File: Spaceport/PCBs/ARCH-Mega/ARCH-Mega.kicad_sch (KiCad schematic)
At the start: 83 parts, among them J10 USB_C_Receptacle_USB2.0_16P, J12 Charge, U4 FT234XD, U5 USBLC6-2P6, U8 BQ25606RGER

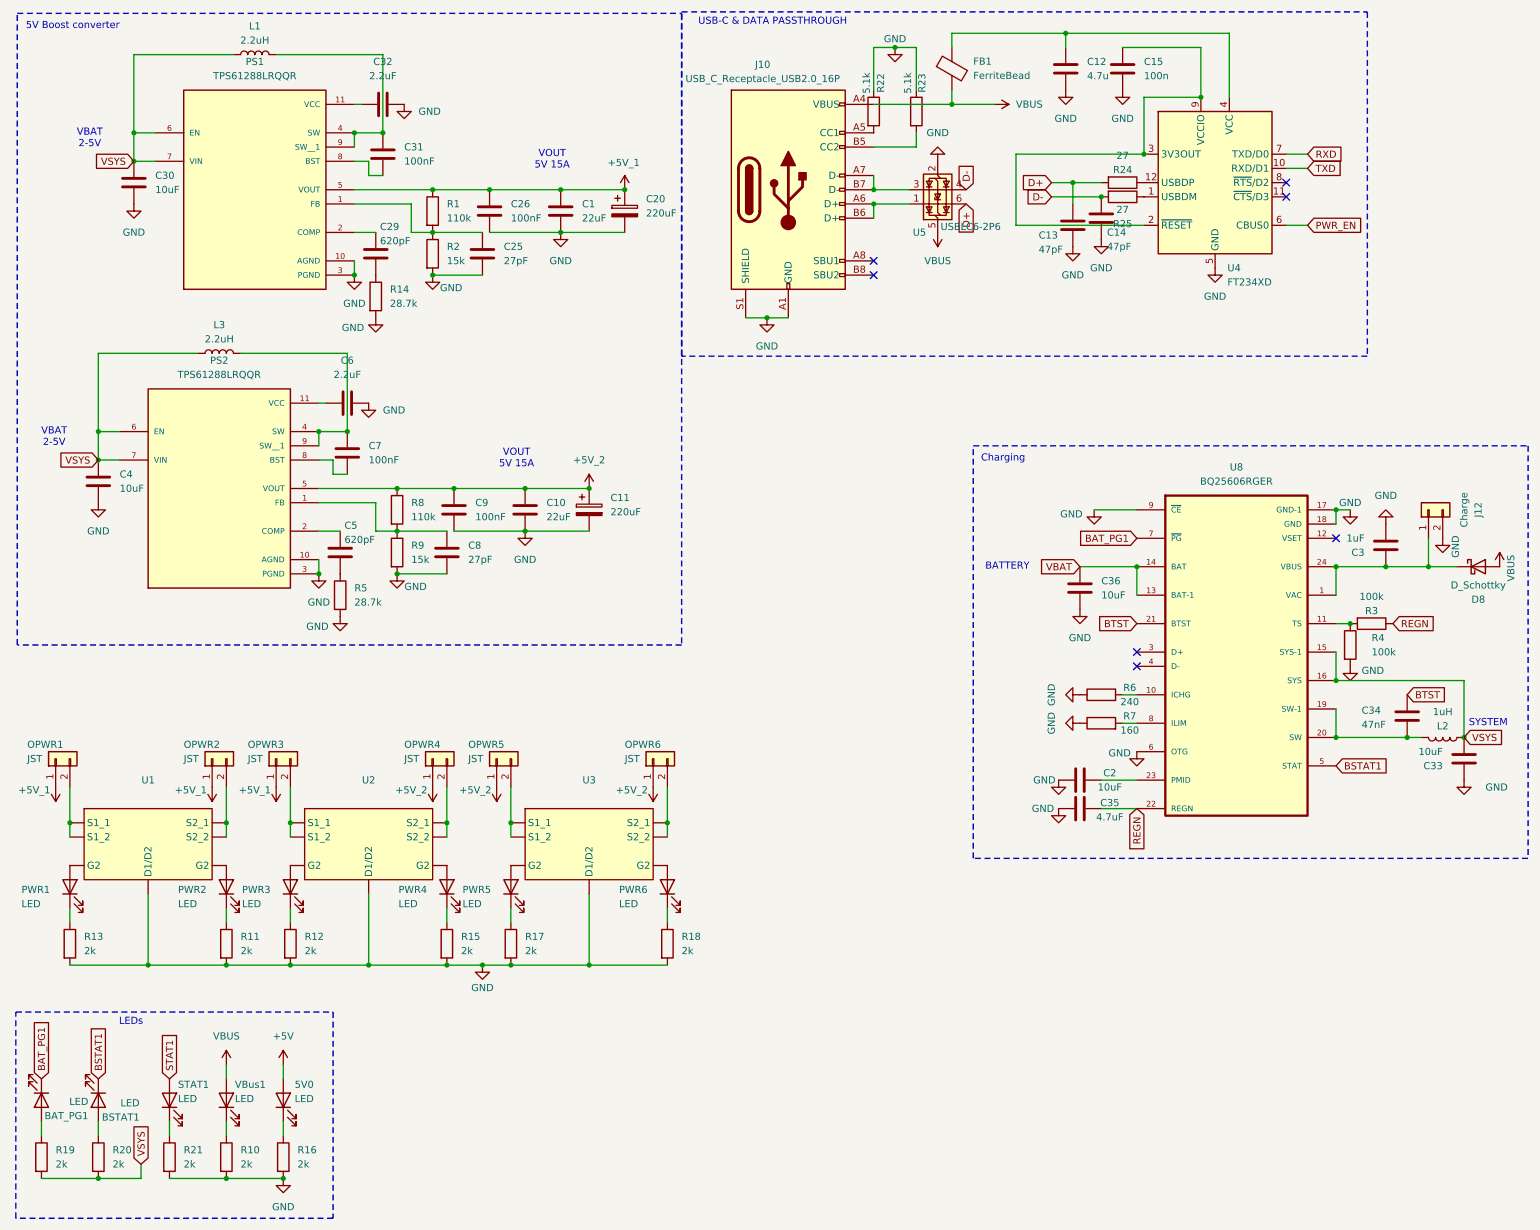
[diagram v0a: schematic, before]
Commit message: initial ARCH-Mega schematic
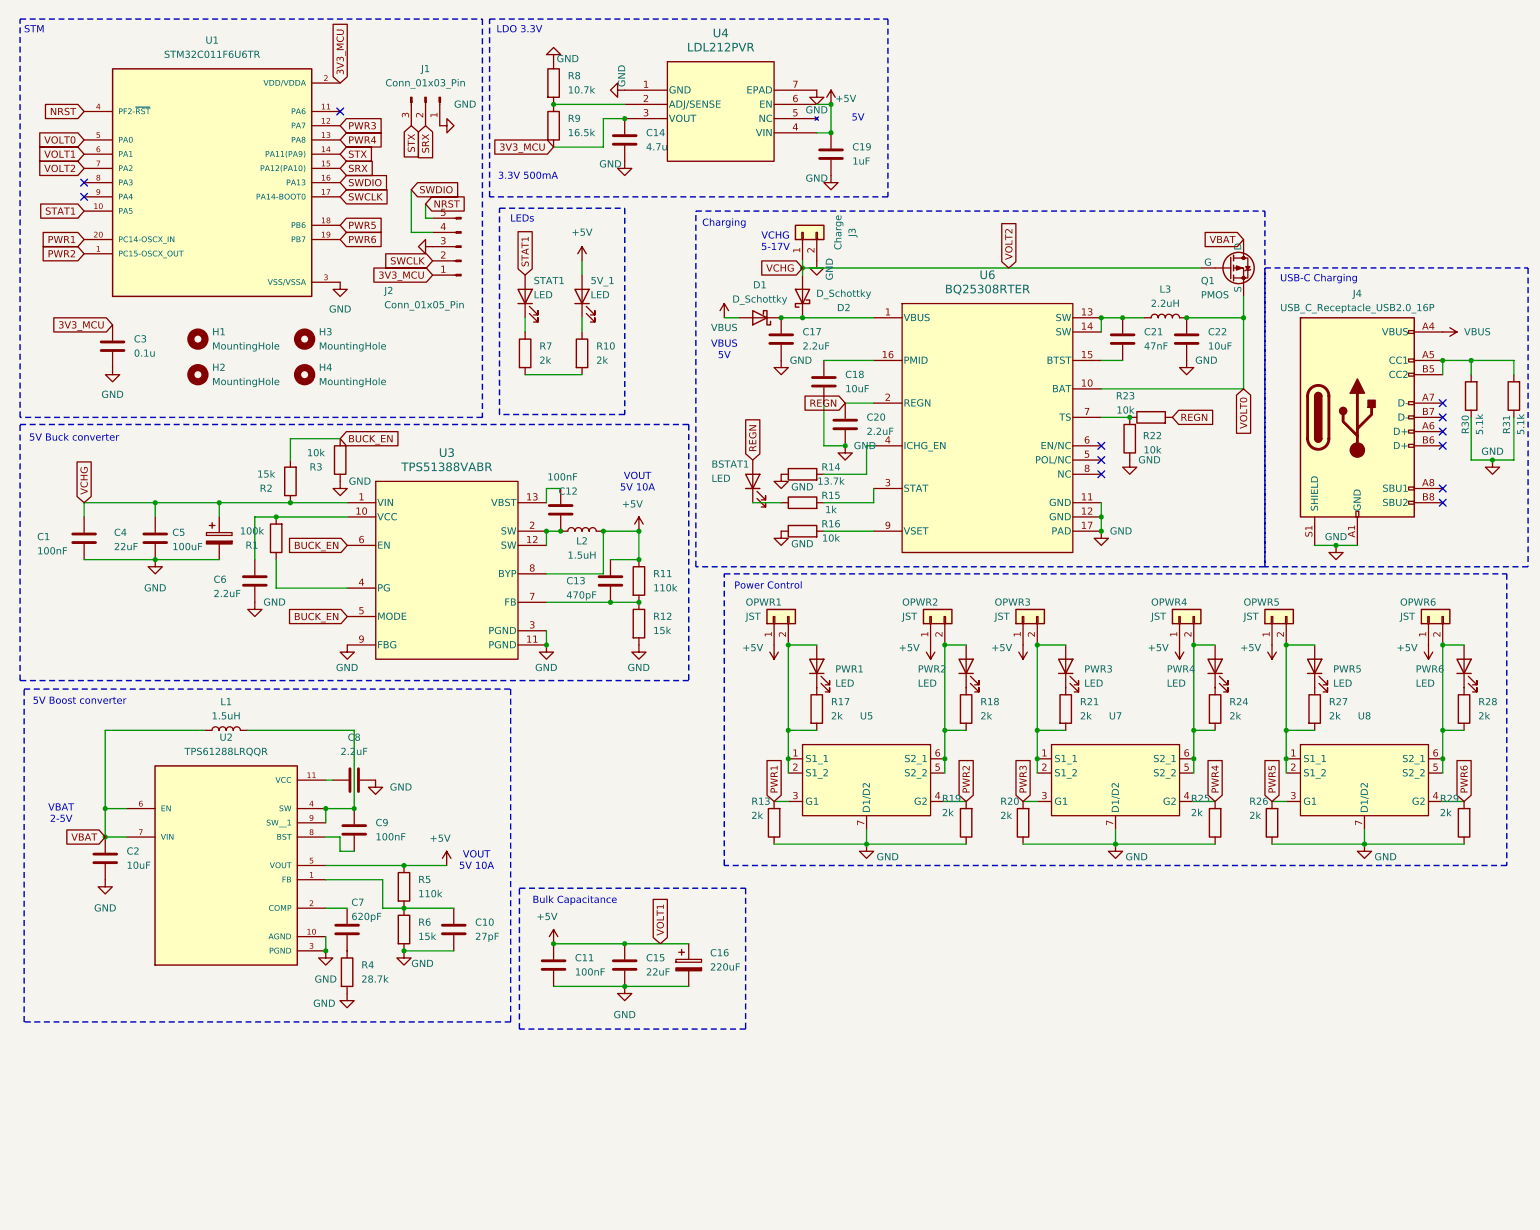
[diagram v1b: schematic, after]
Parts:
- removed 5V0, BAT_PG1: LED, LED_SMD:LED_0805_2012Metric_Pad1.15x1.40mm_HandSolder, symbol Device:LED
- removed C10: 22uF, Capacitor_SMD:C_0805_2012Metric, symbol Device:C
- removed C11: 220uF, Capacitor_THT:CP_Radial_D5.0mm_P2.00mm, symbol Device:C_Polarized
- removed C15: 100n, Capacitor_SMD:C_0805_2012Metric, symbol Device:C
- removed C2, C33, C36: 10uF, Capacitor_SMD:C_0805_2012Metric, symbol Device:C
- removed C34: 47nF, Capacitor_SMD:C_0805_2012Metric, symbol Device:C
- removed C35: 4.7uF, Capacitor_SMD:C_0603_1608Metric, symbol Device:C
- removed C5: 620pF, Capacitor_SMD:C_0603_1608Metric, symbol Device:C
- removed C7, C9: 100nF, Capacitor_SMD:C_0603_1608Metric, symbol Device:C
- removed C8: 27pF, Capacitor_SMD:C_0603_1608Metric, symbol Device:C
- removed FB1: FerriteBead, Resistor_SMD:R_0805_2012Metric_Pad1.20x1.40mm_HandSolder, symbol Device:FerriteBead
- removed J12: Charge, Connector_JST:JST_XH_S2B-XH-A_1x02_P2.50mm_Horizontal, symbol Connector_Generic:Conn_01x02
- removed PS2: TPS61288LRQQR, Avionics:CONV_TPS61288LRQQR, symbol SRAD-Avionics:TPS61288LRQQR
- removed R4: 100k, Resistor_SMD:R_0603_1608Metric, symbol Device:R
- removed R5: 28.7k, Resistor_SMD:R_0603_1608Metric, symbol Device:R
- removed R6: 240, Resistor_SMD:R_0603_1608Metric, symbol Device:R
- removed R7: 160, Resistor_SMD:R_0603_1608Metric, symbol Device:R
- removed U1, U2, U3: ~, symbol Avionics:GSFN0232
- removed U4: FT234XD, Avionics:FT234XD, symbol Interface_USB:FT234XD
- removed U5: USBLC6-2P6, Avionics:USBLC6-2P6, symbol Power_Protection:USBLC6-2P6
- removed U8: BQ25606RGER, Avionics:BQ25606RGER, symbol SRAD-Avionics:BQ25606RGER
- added C1: 100nF, Capacitor_SMD:C_0603_1608Metric, symbol Device:C
- added C17, C20: 2.2uF, Capacitor_SMD:C_0805_2012Metric, symbol Device:C
- added C18, C22: 10uF, Capacitor_SMD:C_0603_1608Metric, symbol Device:C
- added C19: 1uF, Capacitor_SMD:C_0603_1608Metric, symbol Device:C
- added C21: 47nF, Capacitor_SMD:C_0805_2012Metric, symbol Device:C
- added C5: 100uF, Avionics:Wurth_SMD_Cap, symbol Device:C_Polarized
- added D2: D_Schottky, Avionics:Schottky_3A_DO-214AC_SMA, symbol Device:D_Schottky
- added H1, H2, H3, H4: MountingHole, MountingHole:MountingHole_3.2mm_M3, symbol Mechanical:MountingHole
- added J1: Conn_01x03_Pin, Connector_JST:JST_XH_B3B-XH-A_1x03_P2.50mm_Vertical, symbol Connector:Conn_01x03_Pin
- added J2: Conn_01x05_Pin, Connector_PinHeader_2.54mm:PinHeader_1x05_P2.54mm_Vertical, symbol Connector:Conn_01x05_Pin
- added J3: Charge, Connector_JST:JST_XH_S2B-XH-A_1x02_P2.50mm_Horizontal, symbol Connector_Generic:Conn_01x02
- added Q1: PMOS, Avionics:SI7615ADN-T1-GE3, symbol Simulation_SPICE:PMOS
- added R1: 100k, Resistor_SMD:R_0603_1608Metric, symbol Device:R
- added R14: 13.7k, Resistor_SMD:R_0603_1608Metric, symbol Device:R
- added R2: 15k, Resistor_SMD:R_0603_1608Metric, symbol Device:R
- added R21, R26, R27, R28, R29: 2k, Resistor_SMD:R_0603_1608Metric, symbol Device:R
- added R22, R23: 10k, Resistor_SMD:R_0603_1608Metric, symbol Device:R
- added U1: STM32C011F6U6TR, Avionics:STM32C011F6U6TR, symbol Avionics:STM32C011F6U6TR
- added U3: TPS51388VABR, Avionics:TPS513885VABR, symbol Avionics:TPS51388VABR
- added U4: LDL212PVR, Avionics:LDL212PVR, symbol Avionics:LDL212PVR
- added U5, U7, U8: ~, Package_DFN_QFN:DFN-6-1EP_3x2mm_P0.5mm_EP1.65x1.35mm, symbol Avionics:GSFN0232
- added U6: BQ25308RTER, Avionics:BQ25308RTER, symbol Avionics:BQ25308RTER
- C12: value 4.7u -> 100nF; footprint Capacitor_SMD:C_0805_2012Metric -> Capacitor_SMD:C_0603_1608Metric
- C13: value 47pF -> 470pF; footprint Capacitor_SMD:C_0805_2012Metric -> Capacitor_SMD:C_0603_1608Metric
- C14: value 47pF -> 4.7u; footprint Capacitor_SMD:C_0805_2012Metric -> Capacitor_SMD:C_0603_1608Metric
- C16: renamed from C20; footprint Capacitor_THT:CP_Radial_D5.0mm_P2.00mm -> Avionics:Wurth_SMD_Cap
- C2: renamed from C30; footprint Capacitor_SMD:C_0805_2012Metric -> Capacitor_SMD:C_0603_1608Metric
- C3: value 1uF -> 0.1u; footprint Capacitor_SMD:C_0805_2012Metric -> Capacitor_SMD:C_0603_1608Metric
- C4: value 10uF -> 22uF
- L1: value 2.2uH -> 1.5uH
- L2: value 1uH -> 1.5uH
- R11: value 2k -> 110k
- R12: value 2k -> 15k
- R15: value 2k -> 1k
- R16: value 2k -> 10k
- R24, R25: value 27 -> 2k; footprint Resistor_SMD:R_0805_2012Metric -> Resistor_SMD:R_0603_1608Metric
- R3: value 100k -> 10k
- R8: value 110k -> 10.7k
- R9: value 15k -> 16.5k
- renumbered VBus1 to 5V_1, C25 to C10, C26 to C11, C1 to C15, C29 to C7, C32 to C8, C31 to C9, D8 to D1, J10 to J4, R23 to R30, R22 to R31, R14 to R4, R1 to R5, R2 to R6, R21 to R7, PS1 to U2
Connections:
- net +5V_1 is gone; now on net +5V: C11.1, C15.1, C16.1, OPWR1.1 (Pin_1), OPWR2.1 (Pin_1), OPWR3.1 (Pin_1), R5.1, U2.5 (VOUT)
- net +5V: now also 5V_1.2 (A), C13.1, L2.2, OPWR4.1 (Pin_1), OPWR5.1 (Pin_1), OPWR6.1 (Pin_1), R11.1, C19.2, U1.6 (PA1), U3.8 (BYP), U4.4 (VIN), U4.6 (EN)
- net GND: now also C6.1, R13.1, R16.1, R19.1, R20.1, R25.1, R3.1, R8.1, C1.2, C17.1, C18.1, C19.1, C20.1, C22.1, C5.2, J1.1 (Pin_1), J2.3 (Pin_3), J3.2 (Pin_2), R14.1, R22.1, R26.1, R29.1, U1.3 (VSS/VSSA), U3.11 (PGND), U3.3 (PGND), U3.9 (FBG), U4.1 (GND), U4.7 (EPAD), U5.7 (D1/D2), U6.11 (GND), U6.12 (GND), U6.17 (PAD), U7.7 (D1/D2), U8.7 (D1/D2); no longer C12.1, C13.1, C6.2, R10.2, R11.2, R13.2, R15.2, R16.2, R17.2, R18.2, R7.2, R9.2
- net REGN: now also BSTAT1.2 (A), C20.2, R23.2, U6.2 (REGN); no longer R3.1
- net STAT1: now also U1.10 (PA5)
- net VBAT: now also C2.1, L1.1, U2.6 (EN), U2.7 (VIN), Q1.1 (D)
- net VBUS: no longer 5V_1.2 (A)
- net VOLT0: now reaches L3.2
- net VOLT0: now also C22.2, Q1.3 (S), U1.5 (PA0), U6.10 (BAT)
- net at PWR4.2 (A): now also OPWR4.2 (Pin_2), R24.2, U7.5 (S2_2), U7.6 (S2_1)
- net at OPWR3.2 (Pin_2): now also PWR3.2 (A), R21.2, U7.1 (S1_1), U7.2 (S1_2)
- net at OPWR2.2 (Pin_2): now also PWR2.2 (A), R18.2, U5.5 (S2_2), U5.6 (S2_1)
- net at OPWR5.2 (Pin_2): now also PWR5.2 (A), R27.2, U8.1 (S1_1), U8.2 (S1_2)
- net at D1.1 (K): now also C17.2, D2.1 (K), U6.1 (VBUS); no longer C3.1
- net at PWR4.1 (K): now also R24.1; no longer R15.1
- net at C12.2: now also U3.13 (VBST)
- net at R17.1: now also PWR1.1 (K); no longer PWR5.1 (K)
- net BUCK_EN: now reaches R3.2
- net BUCK_EN: now also R2.2, U3.5 (MODE), U3.6 (EN)
- net at OPWR1.2 (Pin_2): now also PWR1.2 (A), R17.2, U5.1 (S1_1), U5.2 (S1_2)
- net at J4.A5 (CC1), R31.2: now also J4.B5 (CC2), R30.2
- net at J4.A6 (D+): no longer J4.B6 (D+)
- net at J4.A7 (D-): no longer J4.B7 (D-)
- net at PWR6.1 (K): now also R28.1; no longer R18.1
- net at PWR6.2 (A): now also OPWR6.2 (Pin_2), R28.2, U8.5 (S2_2), U8.6 (S2_1)
- net at PWR2.1 (K): now also R18.1; no longer R11.1
- net at R8.2, R9.1: now also U4.2 (ADJ/SENSE)
- net at R12.1: now also C13.2, R11.2, U3.7 (FB); no longer PWR3.1 (K)
- removed net +5V_2: OPWR4.1 (Pin_1), OPWR5.1 (Pin_1), OPWR6.1 (Pin_1), R8.1
- net BSTAT1: no longer names the net of BSTAT1.1 (K)
- net BSTAT1: now also R15.1
- removed net D+: C13.2, R24.2
- net D- renamed 3V3_MCU
- net 3V3_MCU: now also C3.1, R9.2, J2.1 (Pin_1), U1.2 (VDD/VDDA), U4.3 (VOUT); no longer R25.2
- removed net VSYS: C2.1, C4.1, L1.1, L2.1, L3.1, R19.2, R20.2, U2.6 (EN), U2.7 (VIN)
- new net: C12.1, L2.1, U3.12 (SW), U3.2 (SW)
- new net: R1.1, U3.4 (PG)
- new net: C6.2, R1.2, U3.10 (VCC)
- new net: R15.2, U6.3 (STAT)
- new net: R10.2, R7.2
- new net: C18.2, U6.16 (PMID)
- new net: R14.2, U6.4 (ICHG_EN)
- new net: PWR3.1 (K), R21.1
- new net: R22.2, R23.1, U6.7 (TS)
- new net: PWR5.1 (K), R27.1
- new net: R16.2, U6.9 (VSET)
- new net: C21.2, L3.1, U6.13 (SW), U6.14 (SW)
- new net: C21.1, U6.15 (BTST)
- new net NRST: J2.5 (Pin_5), U1.4 (PF2-~{RST})
- new net PWR1: R13.2, U1.20 (PC14-OSCX_IN), U5.3 (G1)
- new net PWR2: R19.2, U1.1 (PC15-OSCX_OUT), U5.4 (G2)
- new net PWR3: R20.2, U1.12 (PA7), U7.3 (G1)
- new net PWR4: R25.2, U1.13 (PA8), U7.4 (G2)
- new net PWR5: R26.2, U1.18 (PB6), U8.3 (G1)
- new net PWR6: R29.2, U1.19 (PB7), U8.4 (G2)
- new net SRX: J1.2 (Pin_2), U1.15 (PA12(PA10))
- new net STX: J1.3 (Pin_3), U1.14 (PA11(PA9))
- new net SWCLK: J2.2 (Pin_2), U1.17 (PA14-BOOT0)
- new net SWDIO: J2.4 (Pin_4), U1.16 (PA13)
- new net VCHG: C1.1, C4.1, C5.1, D2.2 (A), J3.1 (Pin_1), Q1.2 (G), R2.1, U1.7 (PA2), U3.1 (VIN)
- no-connect marks 7 -> 12
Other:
- note added: "3.3V 500mA"
- note added: "5V"
- note added: "5V Buck converter"
- note added: "Bulk Capacitance"
- note added: "LDO 3.3V"
- note added: "Power Control"
- note added: "STM"
- note added: "USB-C Charging"
- note added: "VBUS 5V"
- note added: "VCHG 5-17V"
- note added: "VOUT 5V 10A"
- note removed: "BATTERY"
- note removed: "SYSTEM"
- note removed: "USB-C & DATA PASSTHROUGH"
- note removed: "VOUT 5V 15A"
- moved on the sheet: 5V_1, C10, C11, C15, C16, C2, C7, C8, C9, D1, J4, L1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
